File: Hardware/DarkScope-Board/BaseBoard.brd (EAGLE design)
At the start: 108 x 87.6 mm, 90 parts, among them IC1 7805DT, IC2 REG1117, IC3 7905, J1 DCJ0202, Q1 8MHz, T2 9014, U1 STM32F103CBT6, X1 TSW-102-07-G-S, X2 TSW-102-07-G-S, X3 MINI-USB-32005-301, X4 2540-5

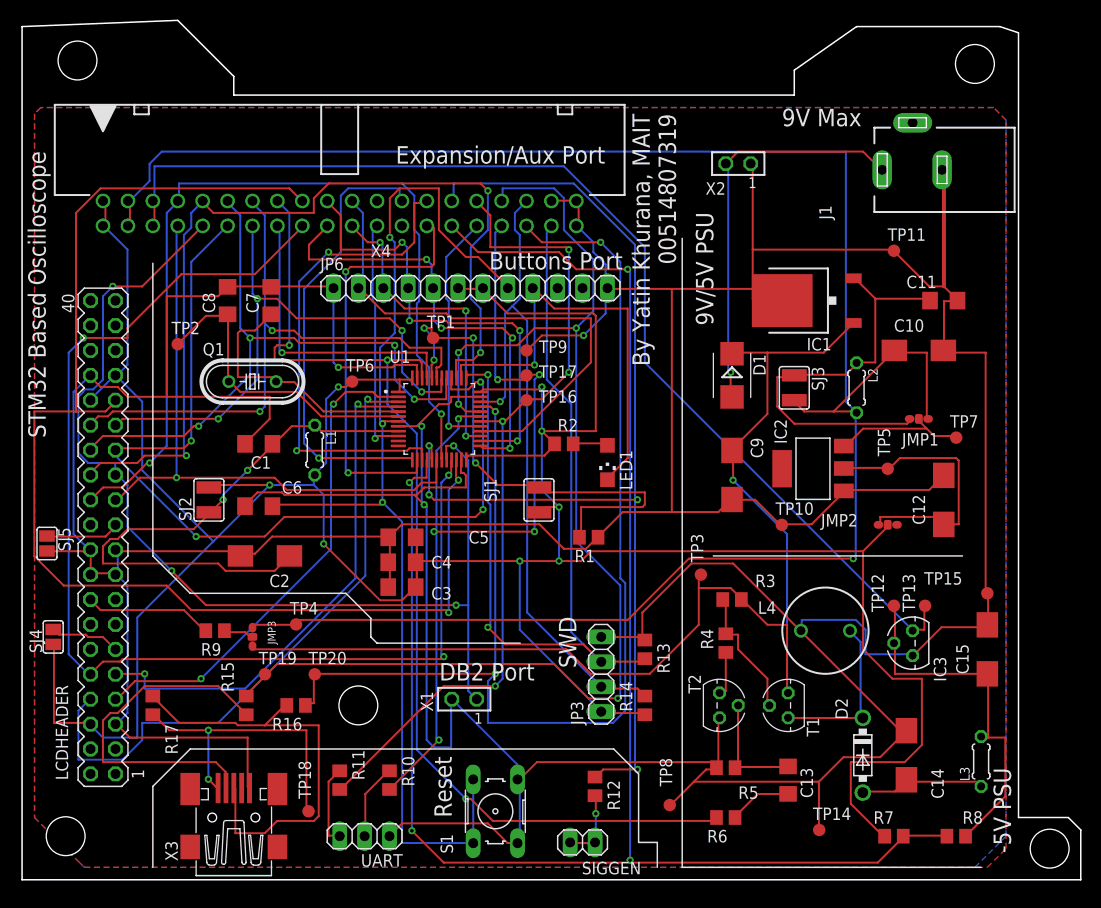
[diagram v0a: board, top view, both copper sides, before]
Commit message: Fixed baseboard
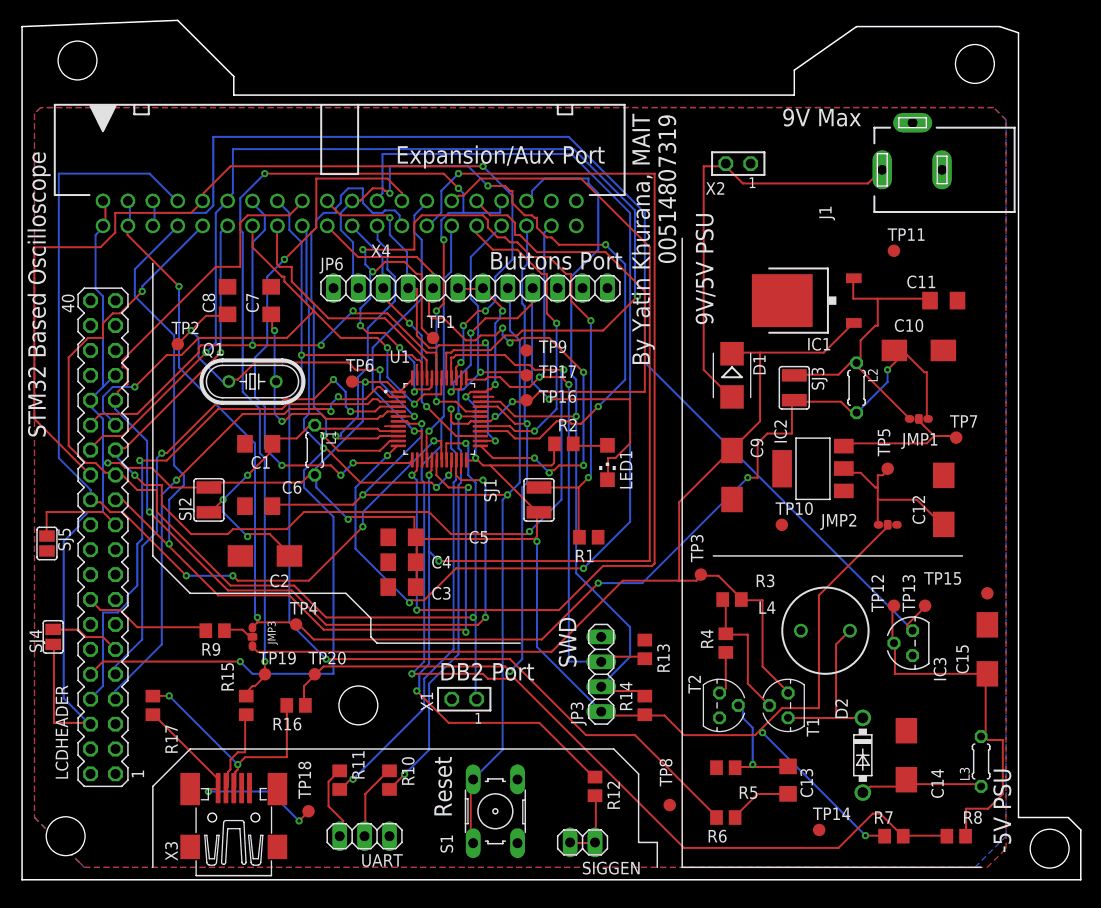
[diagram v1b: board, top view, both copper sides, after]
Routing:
- net GND: track 634.1 -> 5.47 mm, vias 4 -> 0
- net VSENSEL1: track 0.00 -> 110.3 mm, vias 0 -> 3
- net +5V: track 211.5 -> 144.4 mm, vias 1 -> 5
- net ADCIN2: track 42.8 -> 108.4 mm, vias 2 -> 3
- net V-MON: track 176.8 -> 116.8 mm, vias 4 -> 2
- net +3V3: track 334.0 -> 275.8 mm, vias 8 -> 10
- net USBDP: track 127.8 -> 76.2 mm, vias 3 -> 2
- net DB5: track 65.0 -> 114.8 mm, vias 4 -> 2
- net VSENSEL2: track 0.00 -> 45.6 mm, vias 0 -> 1
- net N$21: track 54.0 -> 94.1 mm, vias 4 -> 7
- net DB0: track 62.5 -> 98.7 mm, vias 1 -> 3
- net LCD_NRD: track 121.1 -> 91.5 mm, vias 3 -> 4
- net SWCLK: track 93.0 -> 64.3 mm
- net N$29: track 36.1 -> 8.81 mm
- net LCD_NRESET: track 129.3 -> 103.7 mm, vias 2 -> 3
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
